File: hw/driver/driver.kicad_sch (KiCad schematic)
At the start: 2 parts, among them M1 Stepper_Motor, U1 TMC2209

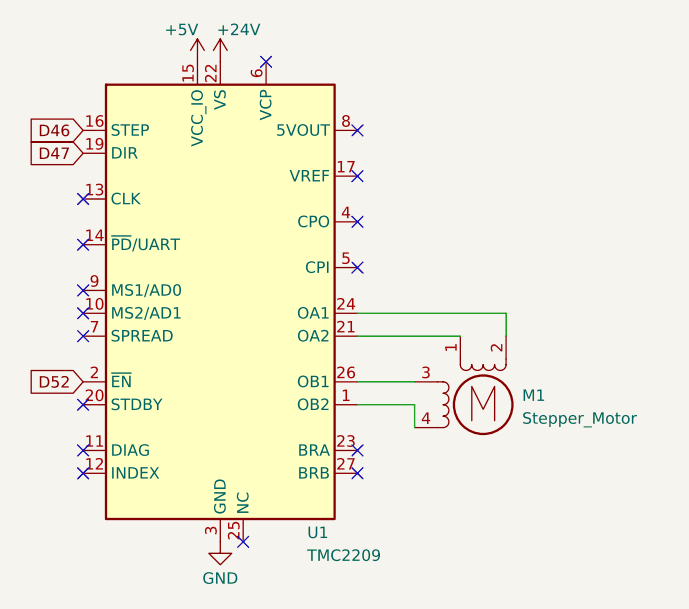
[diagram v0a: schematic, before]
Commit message: update schematics
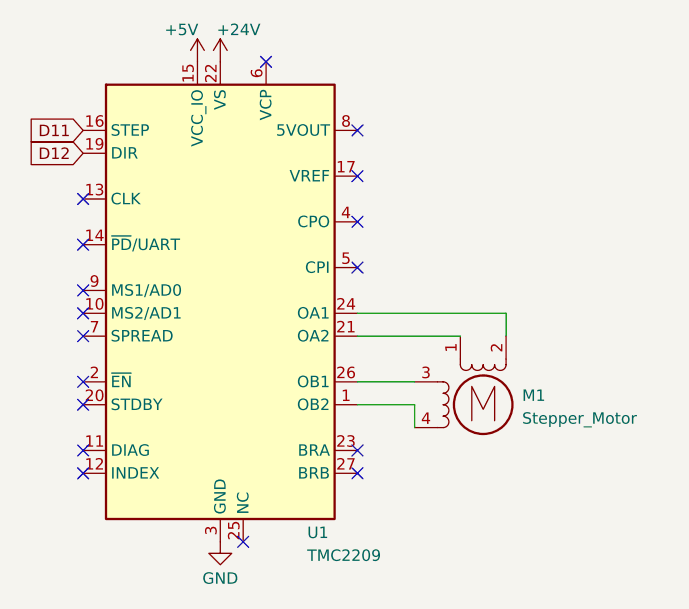
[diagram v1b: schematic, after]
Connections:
- net D46 renamed D11
- net D47 renamed D12
- net D52: no longer names the net of U1.2 (~{EN})
- no-connect marks 16 -> 17
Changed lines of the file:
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@@
+	)
+	(no_connect
+		(at 120.65 99.06)
 	)
 	(no_connect
@@
 		)
 	)
-	(global_label "D47"
+	(global_label "D12"
 		(shape input)
 		(at 120.65 73.66 180)
@@
 		)
 	)
-	(global_label "D46"
+	(global_label "D11"
 		(shape input)
 		(at 120.65 71.12 180)
@@
 			(hide yes)
 			(show_name no)
-			(do_not_autoplace no)
-			(effects
-				(font
-					(size 1.27 1.27)
-				)
-				(justify right)
-			)
-		)
-	)
-	(global_label "D52"
-		(shape input)
-		(at 120.65 99.06 180)
-		(fields_autoplaced yes)
-		(effects
-			(font
-				(size 1.27 1.27)
-			)
-			(justify right)
-		)
-		(property "Intersheetrefs" "${INTERSHEET_REFS}"
-			(at 113.9758 99.06 0)
-			(hide yes)
-			(show_name no)
